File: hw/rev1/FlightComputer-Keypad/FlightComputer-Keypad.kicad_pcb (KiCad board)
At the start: 2 copper layers, 148 x 42 mm, 47 parts, among them J1 Conn_02x20_Odd_Even, J2 Conn_02x10_Odd_Even, SW1 SW_Push, SW2 SW_Push, SW3 SW_Push, SW4 SW_Push, SW5 SW_Push, SW6 SW_Push, SW7 SW_Push, SW8 SW_Push, SW9 SW_Push

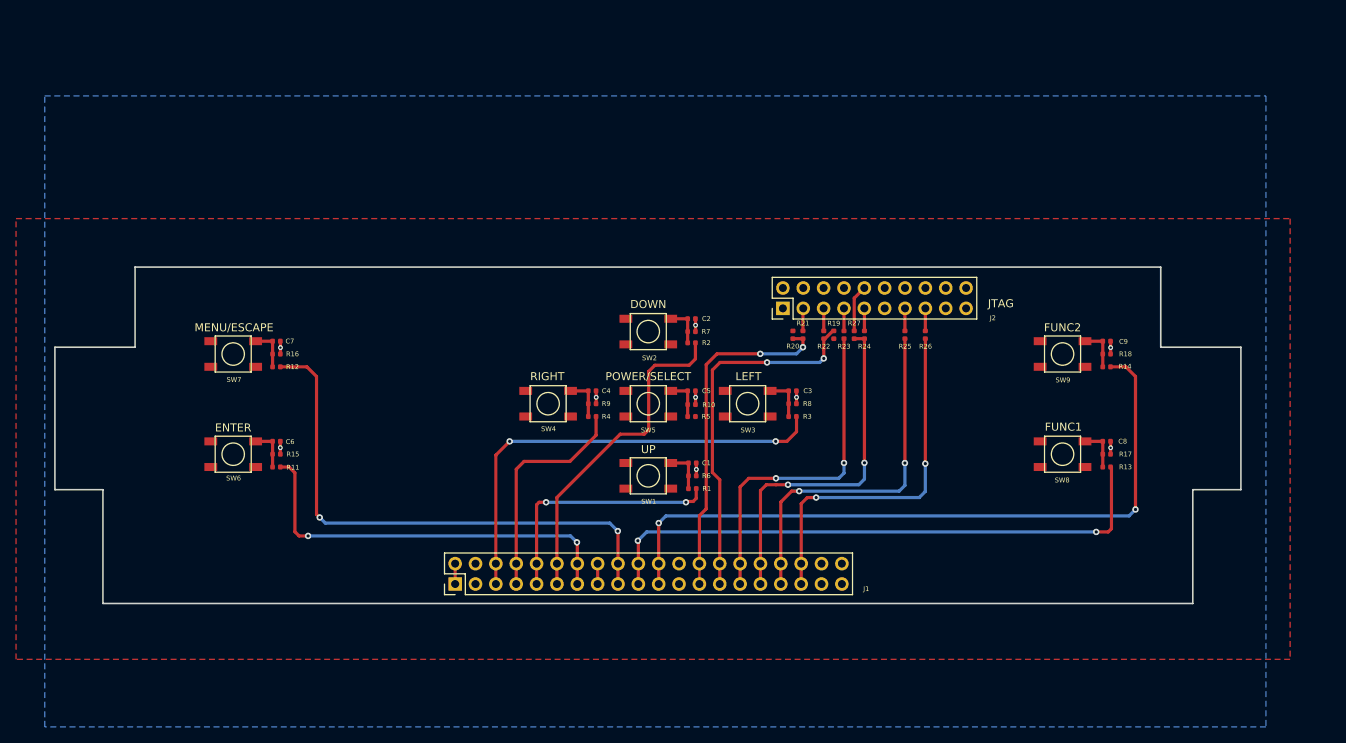
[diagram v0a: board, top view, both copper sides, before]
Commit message: ...
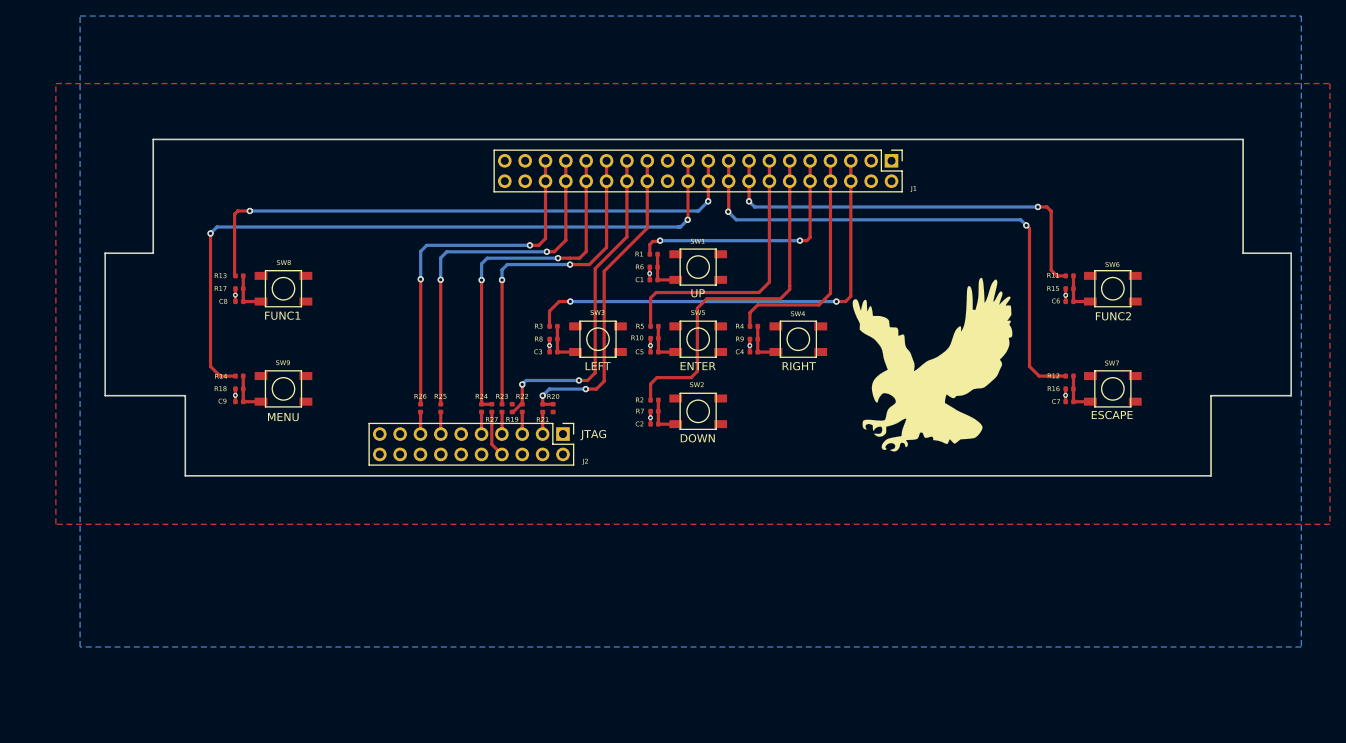
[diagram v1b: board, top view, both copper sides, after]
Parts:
- added G***: LOGO, FlightComputer_Library:LOGO-EAGLE-02, F.Cu at (179.4, 93.2)
- moved SW6 111.7 mm to (201.9, 83.8), turned to 180 degrees
- moved R13 110.8 mm to (92.9, 82.2), turned to 180 degrees
- moved R17 110.2 mm to (92.9, 83.8), turned to 0 degrees
- moved SW7 109.9 mm to (201.9, 96.2), turned to 180 degrees
- moved C8 109.6 mm to (92.9, 85.3), turned to 180 degrees
- moved C9 108.5 mm to (92.9, 97.8), turned to 180 degrees
- moved R18 108.3 mm to (92.9, 96.2), turned to 0 degrees
- moved R14 108.2 mm to (92.9, 94.7), turned to 180 degrees
- moved R11 101.8 mm to (196.5, 82.2), turned to 180 degrees
- moved R15 101.1 mm to (196.5, 83.8), turned to 0 degrees
- moved C6 100.5 mm to (196.5, 85.3), turned to 180 degrees
- moved SW8 99.4 mm to (98.4, 83.8), turned to 180 degrees
- moved C7 99.3 mm to (196.5, 97.8), turned to 180 degrees
- moved R16 99.1 mm to (196.5, 96.2), turned to 0 degrees
- moved R12 99.0 mm to (196.5, 94.7), turned to 180 degrees
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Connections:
- J1 pad 23: (no net) -> Net-(J1-Pad23)
- J1 pad 24: (no net) -> Net-(J1-Pad24)
- J1 pad 3: (no net) -> Net-(J1-Pad3)
- J1 pad 37: (no net) -> Net-(J1-Pad37)
- J1 pad 38: (no net) -> Net-(J1-Pad38)
- J1 pad 4: (no net) -> Net-(J1-Pad4)
- J2 pad 11: (no net) -> Net-(J2-Pad11)
- J2 pad 17: (no net) -> Net-(J2-Pad17)
- J2 pad 19: (no net) -> Net-(J2-Pad19)
- R11 pad 2: /KEY_ENTER -> /KEY_MENU
- R5 pad 2: (no net) -> /KEY_ENTER
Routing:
- net /KEY_MENU: track 2.54 -> 52.7 mm, vias 0 -> 2
- net /KEY_ENTER: track 50.4 -> 34.3 mm, vias 2 -> 0
- net /TDI: track 45.7 -> 41.9 mm
- net /KEY_DOWN: track 41.5 -> 44.9 mm
- net VCC_MCU: track 2.54 -> 0.00 mm
- net /TRST: track 43.0 -> 40.6 mm
- net /TDO: track 45.8 -> 44.7 mm
- net /KEY_RIGHT: track 28.4 -> 29.3 mm
- net /TMS: track 42.6 -> 41.8 mm
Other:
- outline, holes or cut-outs redrawn
- board text added: "ESCAPE"
- board text added: "MENU"
- board text removed: "MENU/ESCAPE"
- board text removed: "POWER/SELECT"
